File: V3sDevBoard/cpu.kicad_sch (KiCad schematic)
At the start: 31 parts, among them U1 Allwinner_V3s, Y1 32768, Y2 24M

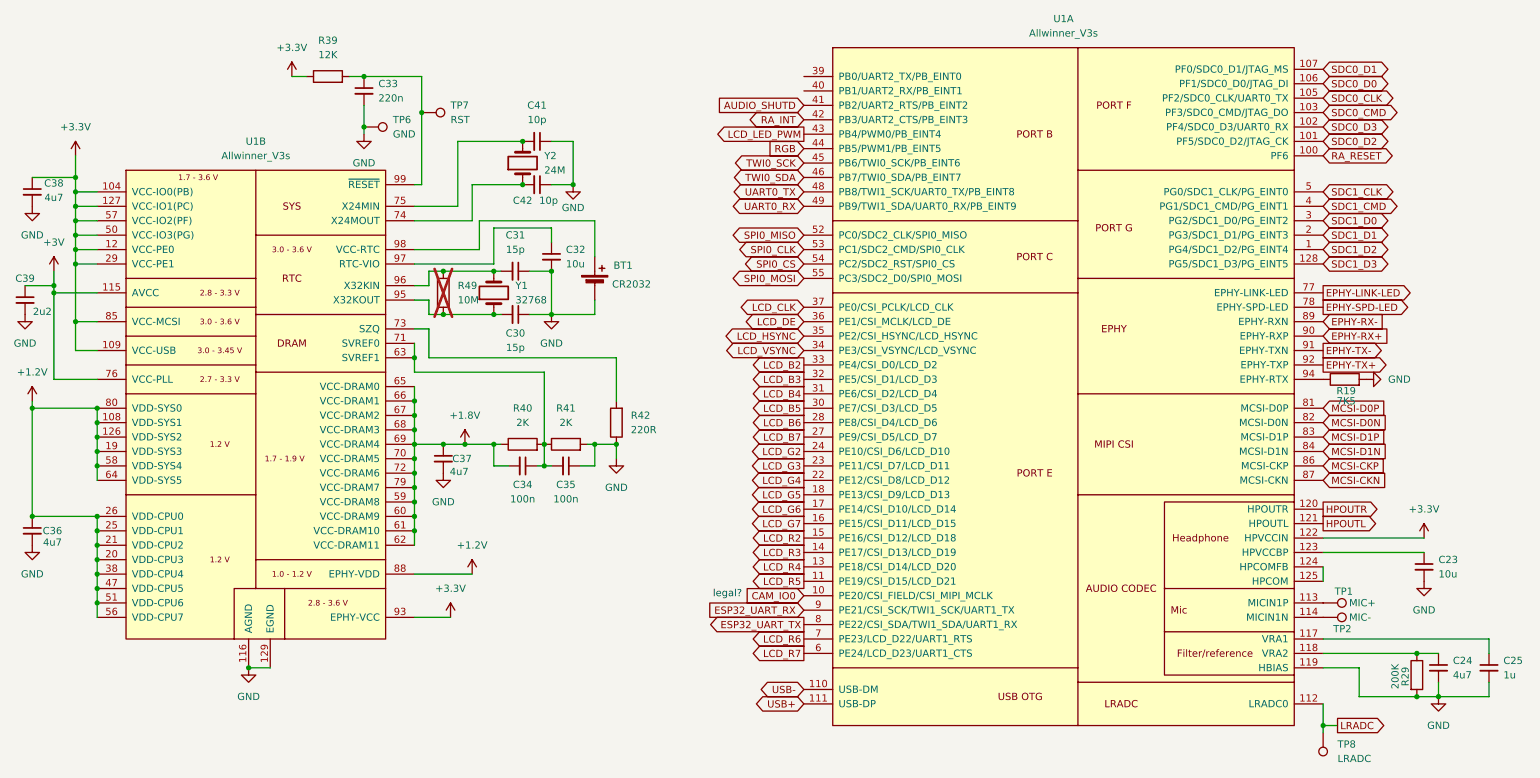
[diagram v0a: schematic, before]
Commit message: completing schematics
completing schematics, adding netclasses, fixing bugs, updating readme, starting pcb
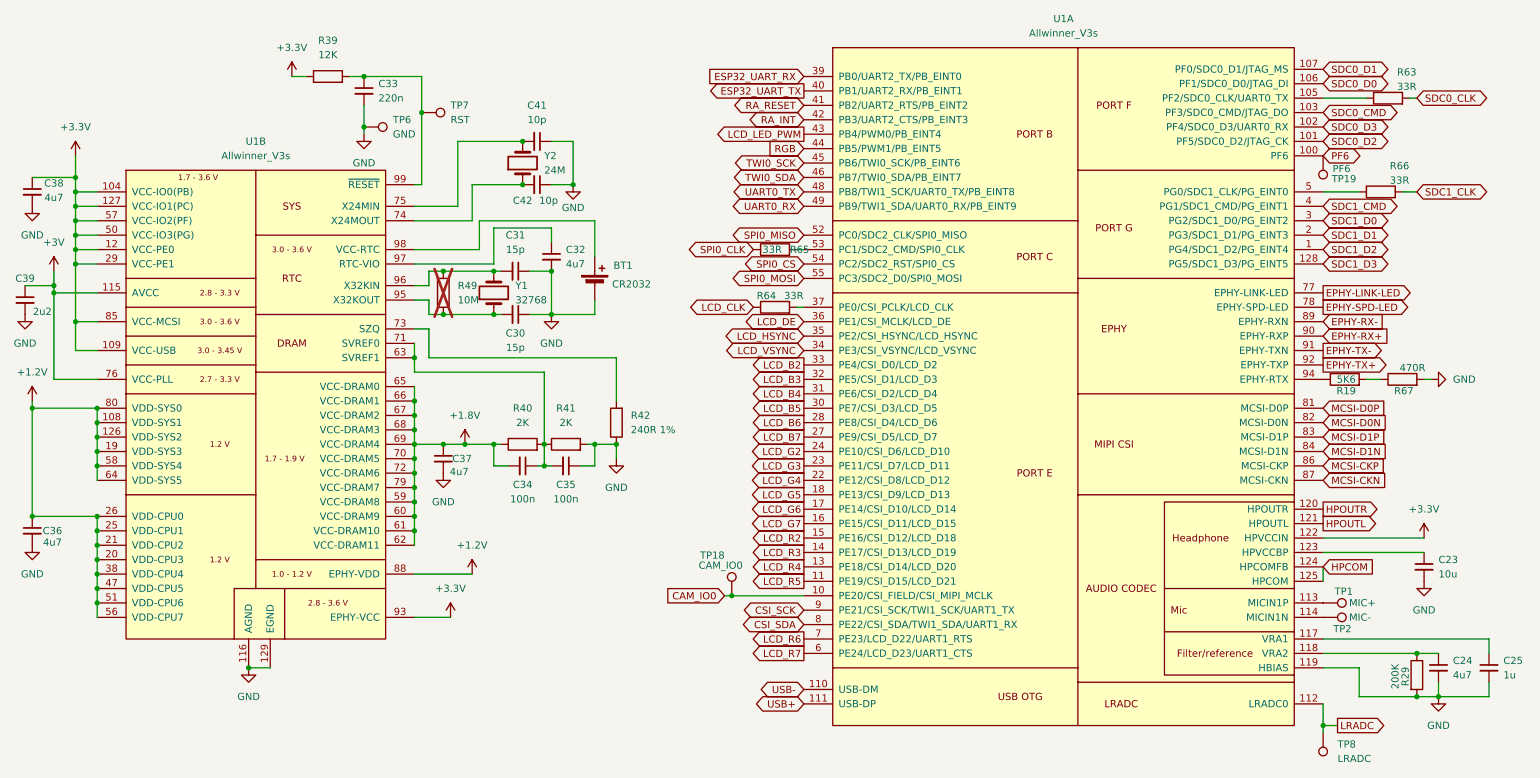
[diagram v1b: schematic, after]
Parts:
- added R63, R64, R65, R66: 33R, Resistor_SMD:R_0603_1608Metric_Pad0.98x0.95mm_HandSolder, symbol Device:R
- added R67: 470R, Resistor_SMD:R_0603_1608Metric_Pad0.98x0.95mm_HandSolder, symbol Device:R
- added TP18: CAM_IO0, TestPoint:TestPoint_Pad_D1.0mm, symbol Connector:TestPoint
- added TP19: PF6, TestPoint:TestPoint_Pad_D1.0mm, symbol Connector:TestPoint
- C32: value 10u -> 4u7
- R19: value 7K5 -> 5K6; footprint Resistor_SMD:R_0805_2012Metric_Pad1.20x1.40mm_HandSolder -> Resistor_SMD:R_0603_1608Metric_Pad0.98x0.95mm_HandSolder
- R42: value 220R -> 240R 1%
- TP1, TP2: footprint TestPoint:TestPoint_Pad_D1.0mm -> TestPoint:TestPoint_Pad_1.0x1.0mm
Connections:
- net AUDIO_SHUTD is gone; now on net RA_RESET: U1.41 (PB2/UART2_RTS/PB_EINT2)
- net CAM_IO0: now also TP18.1
- net ESP32_UART_RX: now also U1.39 (PB0/UART2_TX/PB_EINT0); no longer U1.9 (PE21/CSI_SCK/TWI1_SCK/UART1_TX)
- net ESP32_UART_TX: now also U1.40 (PB1/UART2_RX/PB_EINT1); no longer U1.8 (PE22/CSI_SDA/TWI1_SDA/UART1_RX)
- net GND: now also R67.2; no longer R19.2
- net LCD_CLK: now also R64.1; no longer U1.37 (PE0/CSI_PCLK/LCD_CLK)
- net RA_RESET: no longer U1.100 (PF6)
- net SDC0_CLK: now also R63.2; no longer U1.105 (PF2/SDC0_CLK/UART0_TX)
- net SDC1_CLK: now also R66.2; no longer U1.5 (PG0/SDC1_CLK/PG_EINT0)
- net SPI0_CLK: now also R65.1; no longer U1.53 (PC1/SDC2_CMD/SPI0_CLK)
- net at C41.2, U1.75 (X24MIN): now also Y2.2; no longer Y2.4 (2)
- net HPCOM: now reaches U1.124 (HPCOMFB), U1.125 (HPCOM)
- new net: R64.2, U1.37 (PE0/CSI_PCLK/LCD_CLK)
- new net: R63.1, U1.105 (PF2/SDC0_CLK/UART0_TX)
- new net: R66.1, U1.5 (PG0/SDC1_CLK/PG_EINT0)
- new net: R65.2, U1.53 (PC1/SDC2_CMD/SPI0_CLK)
- new net: R19.2, R67.1
- new net CSI_SCK: U1.9 (PE21/CSI_SCK/TWI1_SCK/UART1_TX)
- new net CSI_SDA: U1.8 (PE22/CSI_SDA/TWI1_SDA/UART1_RX)
- new net PF6: TP19.1, U1.100 (PF6)
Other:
- note removed: "legal?"
- company: J.K. -> jakub.kmiecik@protonmail.com
